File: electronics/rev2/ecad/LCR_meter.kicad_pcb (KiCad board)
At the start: 2 copper layers, 57 parts, among them J1 DUT, J2 DUT, J3 SWITCH, J4 SWITCH, U1 OP179GRT, U2 MCP6001R, U3 LM6144xIx, U4 74HC4051, U5 SC0915, U6 LM6144xIx, U7 LM4040DBZ-3

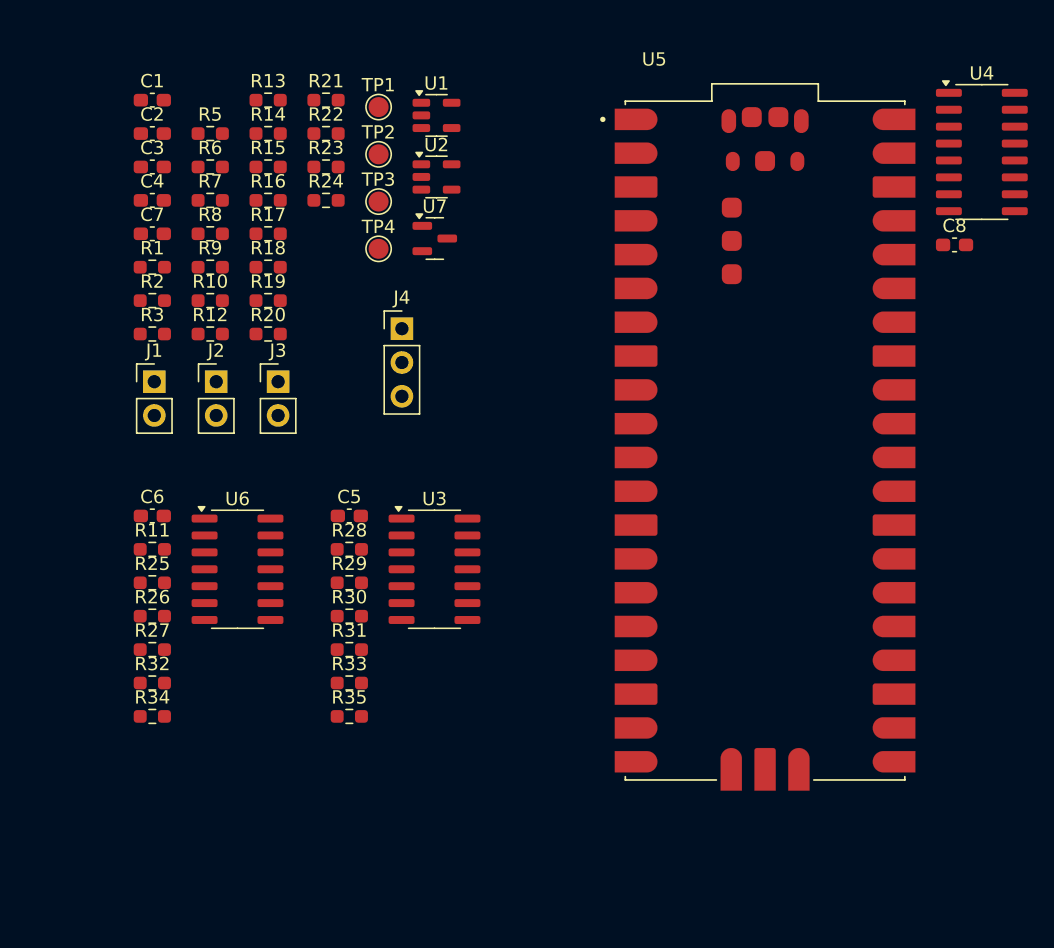
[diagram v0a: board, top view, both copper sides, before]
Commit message: rev2 design work
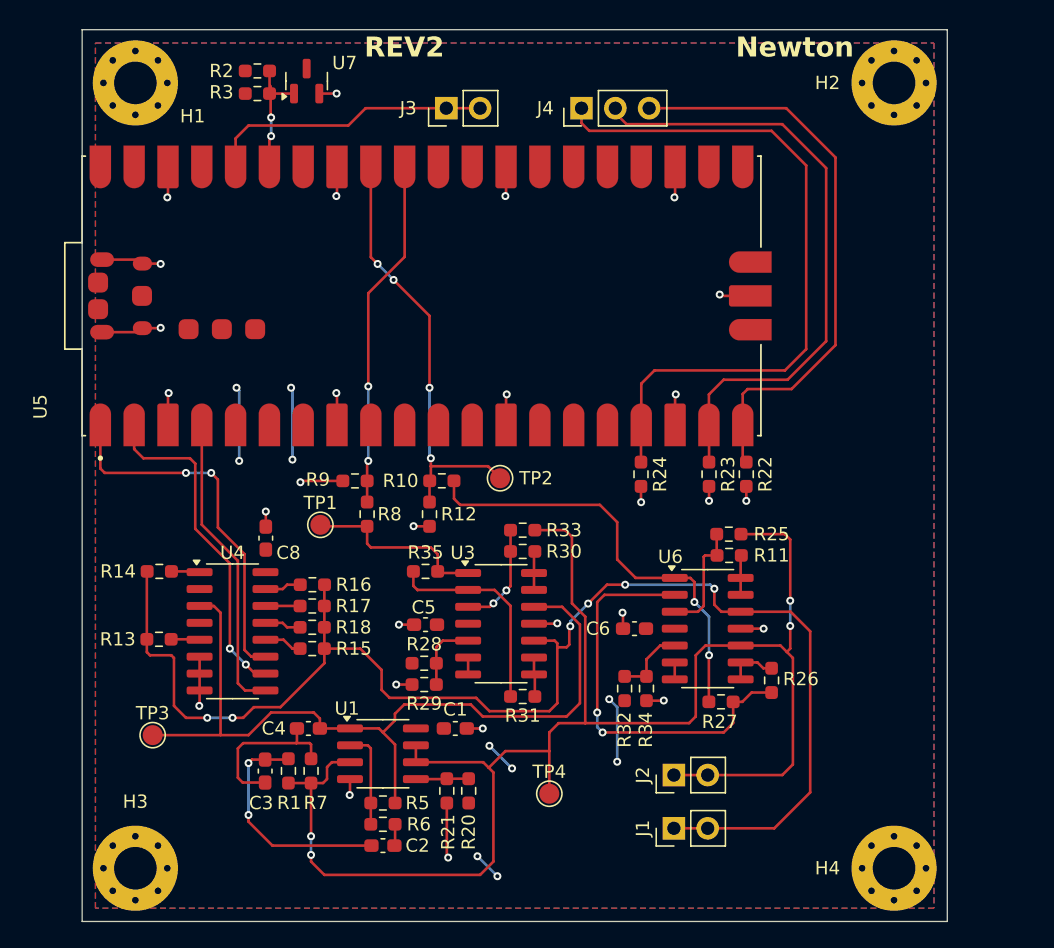
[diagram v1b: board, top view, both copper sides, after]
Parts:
- removed C7: 0.1uF, Capacitor_SMD:C_0603_1608Metric_Pad1.08x0.95mm_HandSolder
- removed R19: 49.9, Resistor_SMD:R_0603_1608Metric_Pad0.98x0.95mm_HandSolder
- removed U2: MCP6001R, Package_TO_SOT_SMD:SOT-23-5
- added H1: M3, MountingHole:MountingHole_3.2mm_M3_Pad_Via, F.Cu at (124.0, 74.0)
- added H2: M3, MountingHole:MountingHole_3.2mm_M3_Pad_Via, F.Cu at (181.0, 74.0)
- added H3: M3, MountingHole:MountingHole_3.2mm_M3_Pad_Via, F.Cu at (124.0, 133.0)
- added H4: M3, MountingHole:MountingHole_3.2mm_M3_Pad_Via, F.Cu at (181.0, 133.0)
- J4: value SWITCH -> INPUT SWITCH
- R1, R6, R7: value 6.49k -> 6.49k+/-0.1%
- R10, R8: value 6.81k -> 6.81k+/-0.1%
- R12, R20, R21, R9: value 10k -> 10k+/-0.1%
- R13: value 49.9M -> 49.9M+/-0.1%
- R14: value 4.99M -> 4.99M+/-0.1%
- R15: value 499k -> 499k+/-0.1%
- R16: value 49.9k -> 49.9k+/-0.1%
- R17: value 4.99k -> 4.99k+/-0.1%
- R18: value 499 -> 499+/-0.1%
- R5: value 249k -> 249k+/-0.1%
- U1: value OP179GRT -> MCP6002-xSN; footprint Package_TO_SOT_SMD:SOT-23-5 -> Package_SO:SOIC-8_3.9x4.9mm_P1.27mm
- moved U4 66.8 mm to (131.3, 115.2)
- moved C8 56.2 mm to (133.8, 108.2), turned to -90 degrees
- moved C2 56.2 mm to (142.6, 131.3), turned to 180 degrees
- moved R21 52.7 mm to (147.4, 127.2), turned to -90 degrees
- moved C1 52.4 mm to (148.0, 122.5)
- moved R5 51.9 mm to (142.6, 128.1)
- moved J1 51.5 mm to (164.5, 130.0), turned to 90 degrees
- moved R6 51.1 mm to (142.6, 129.7)
- moved U1 48.1 mm to (142.6, 124.4)
- moved R26 46.8 mm to (171.8, 118.9), turned to -90 degrees
- moved C3 46.2 mm to (133.8, 125.7), turned to -90 degrees
- moved J2 45.3 mm to (164.5, 126.0), turned to 90 degrees
- moved TP3 43.5 mm to (125.3, 123.0)
- moved R7 43.5 mm to (137.2, 125.7), turned to -90 degrees
- moved R25 43.5 mm to (168.6, 107.9), turned to 180 degrees
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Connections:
- J2 pad 1: /DiffAmp2/IN- -> /DiffAmp1/REF
- J2 pad 2: /DiffAmp2/IN- -> /DiffAmp1/REF
- R1 pad 2: /DiffAmp2/IN- -> /DiffAmp1/REF
- R13 pad 1: Net-(U4-A6) -> Net-(U4-A5)
- R14 pad 1: Net-(U4-A5) -> Net-(U4-A4)
- R15 pad 1: Net-(U4-A4) -> Net-(U4-A3)
- R16 pad 1: Net-(U4-A3) -> Net-(U4-A2)
- R17 pad 1: Net-(U4-A2) -> Net-(U4-A1)
- R18 pad 1: Net-(U4-A1) -> Net-(U4-A0)
- R20 pad 2: Net-(U1-+) -> Net-(U1B-+)
- R21 pad 1: Net-(U1-+) -> Net-(U1B-+)
- R25 pad 1: GND -> /DiffAmp1/REF
- R33 pad 1: GND -> /DiffAmp1/REF
- R5 pad 1: Net-(U2--) -> Net-(U1A--)
- R6 pad 1: Net-(U2--) -> Net-(U1A--)
- R7 pad 2: /DiffAmp2/IN- -> /DiffAmp1/REF
- R8 pad 1: /DiffAmp1/OUT -> Net-(U5-GP26)
- R8 pad 2: Net-(U5-GP26) -> /DiffAmp1/OUT
- TP1 pad 1: Net-(U5-GP26) -> /DiffAmp1/OUT
- TP4 pad 1: /DiffAmp2/IN- -> /DiffAmp1/REF
- U1 pad 1: /DiffAmp2/IN- -> /DiffAmp1/IN+
- U1 pad 2: +5V -> Net-(U1A--)
- U1 pad 3: Net-(U1-+) -> /DiffAmp1/REF
- U1 pad 4: /DiffAmp2/IN- -> GND
- U1 pad 5: GND -> Net-(U1B-+)
- U4 pad 2: Net-(U4-A6) -> unconnected-(U4-A6-Pad2)
- U6 pad 10: /DiffAmp2/IN- -> /DiffAmp1/REF
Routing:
- net /DiffAmp1/REF: track 0.00 -> 121.2 mm, vias 0 -> 4
- net /DiffAmp1/IN-: track 0.00 -> 105.6 mm, vias 0 -> 6
- net /DiffAmp1/IN+: track 0.00 -> 62.4 mm
- net GND: track 0.00 -> 58.7 mm, vias 0 -> 28
- net Net-(J4-Pin_1): track 0.00 -> 52.5 mm
- net Net-(J4-Pin_2): track 0.00 -> 46.5 mm
- net Net-(J4-Pin_3): track 0.00 -> 43.4 mm
- net /DiffAmp2/OUT: track 0.00 -> 33.1 mm, vias 0 -> 2
- net Net-(U5-GP27): track 0.00 -> 32.7 mm, vias 0 -> 4
- net Net-(U6A--): track 0.00 -> 30.9 mm, vias 0 -> 2
- net /bit0: track 0.00 -> 27.9 mm, vias 0 -> 2
- net Net-(U5-GP26): track 0.00 -> 26.3 mm, vias 0 -> 2
- net /bit1: track 0.00 -> 25.3 mm, vias 0 -> 2
- net /bit2: track 0.00 -> 22.8 mm
- net +3.3V: track 0.00 -> 21.5 mm
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- added copper zone on F.Cu, net +5V
- added copper zone on B.Cu, net GND
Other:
- board outline added: 65 x 67 mm
- board text added: "Newton"
- board text added: "REV2"
